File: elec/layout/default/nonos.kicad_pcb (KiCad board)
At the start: 4 copper layers, 45 x 122 mm, 75 parts, among them CN1 HRSHirose_DF40C_100DS_0_4V51, CN2 HRSHirose_DF40C_100DS_0_4V51, Q1 MOSFET, U1 STUSB4500QTR, U2 _Texas_Instruments_SN74LVC1G0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, U3 _Texas_Instruments_TAS5825MRH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, U4 _HCTL_HC_TYPE_C_24P_VS9_3_5A_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, U5 JST_Sales_America_B02B_XASK_1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, U6 JST_Sales_America_B02B_XASK_1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, U7 _Texas_Instruments_TPS56637RP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

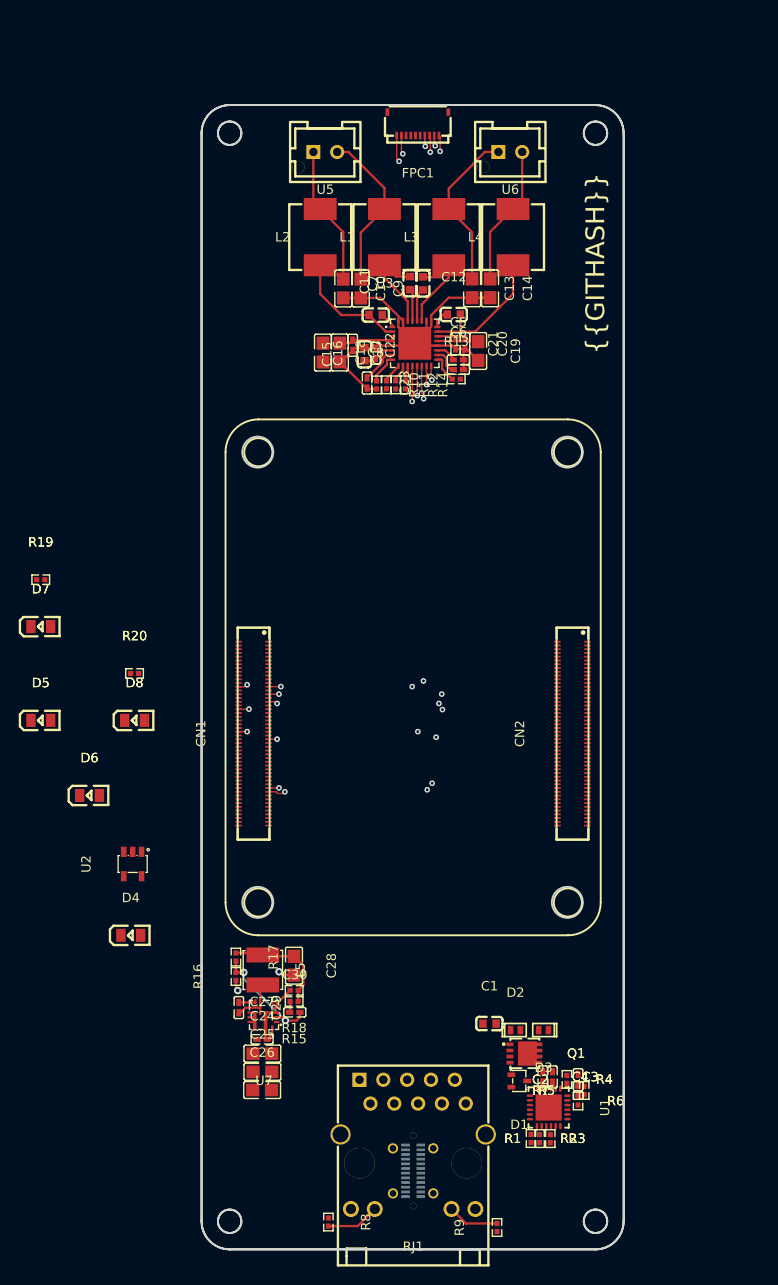
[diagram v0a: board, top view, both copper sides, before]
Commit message: layout 95%
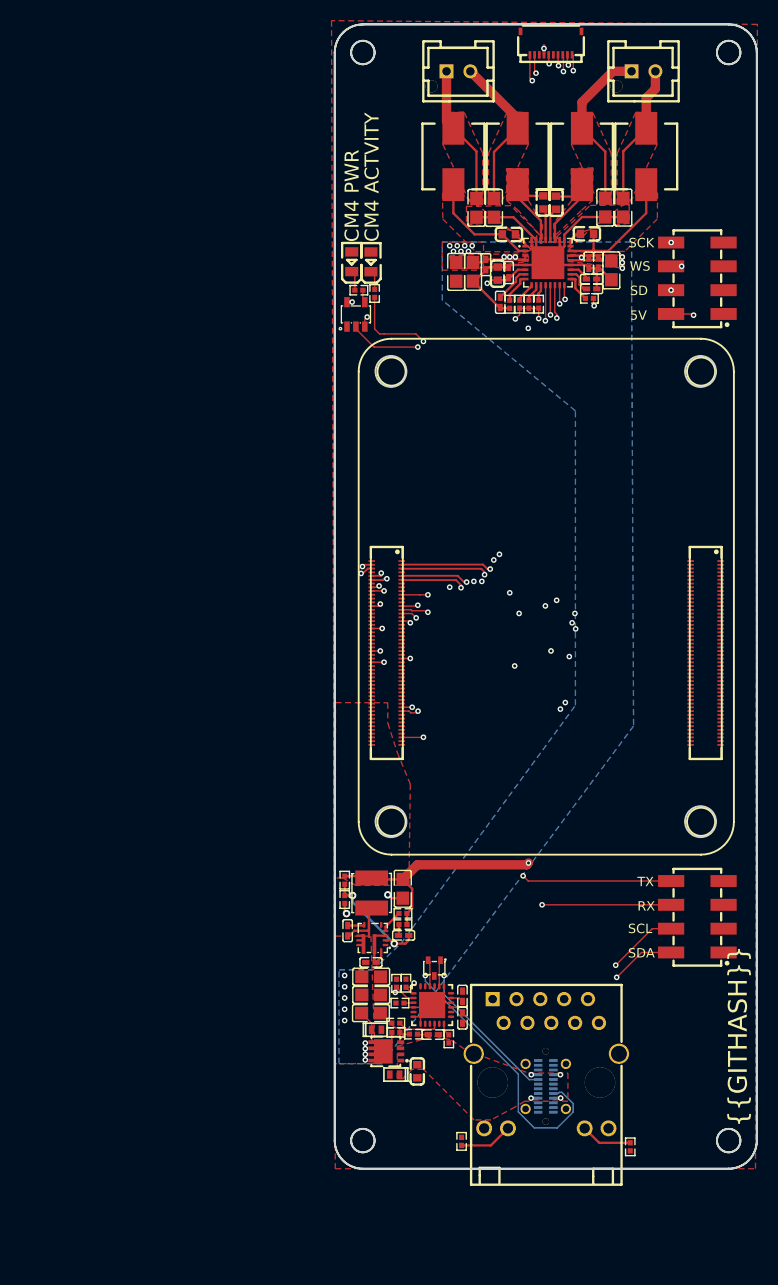
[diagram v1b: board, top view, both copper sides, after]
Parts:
- removed D6, D7, D8: , lcsc:LED0805-R-RD
- added HDR1: HCTL_PZ254_2_04_S, lcsc:HDR-SMD_8P-P2.54-V-M-R2-C4-LS7.4, F.Cu at (169.4, 130.9)
- added HDR2: HCTL_PZ254_2_04_S, lcsc:HDR-SMD_8P-P2.54-V-M-R2-C4-LS7.4, F.Cu at (169.4, 62.9)
- C2: value 100nF ±10% 16V X7R -> 1µF ±10% 25V X5R
- C4: value 1µF ±10% 25V X5R -> 100nF ±10% 16V X7R
- moved D4 76.2 mm to (134.6, 61.1), turned to 90 degrees
- moved U2 63.2 mm to (133.0, 66.7), turned to -90 degrees
- moved D5 59.1 mm to (132.6, 61.1), turned to 90 degrees
- moved R20 47.3 mm to (133.3, 64.1)
- moved R19 46.9 mm to (135.0, 64.5), turned to -90 degrees
- moved R3 22.5 mm to (137.3, 138.0), turned to 90 degrees
- moved R1 21.6 mm to (137.7, 140.1), turned to 0 degrees
- moved R2 21.3 mm to (138.3, 138.0), turned to 90 degrees
- moved R6 21.1 mm to (137.3, 142.3), turned to 0 degrees
- moved R5 21.0 mm to (137.3, 143.3), turned to 180 degrees
- moved R7 18.6 mm to (139.1, 143.5), turned to 0 degrees
- moved D3 17.8 mm to (135.2, 143.0), turned to 0 degrees
- moved U4 16.8 mm to (153.2, 149.0)
- moved C23 16.6 mm to (148.4, 65.4)
- moved R11 16.6 mm to (150.5, 65.6)
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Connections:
- net pd_controller.PD_CONTROLLER-signal renamed pd_controller.pd_controller-signal-1
- net pd_controller.PD_CONTROLLER-signal-1 renamed pd_controller.pd_controller-signal
- net pd_controller.PD_CONTROLLER.footprint.pins[18].net-net renamed pd_controller.pd_controller.footprint.pins[18].net-net
- net pins[40] renamed processor.hdi_b-pins[40]
- net pins[46] renamed processor-pins[46]-1
- net pins[49] renamed processor.hdi_b-pins[49]
- net processor-signal-8 renamed processor-pins[49]
- net processor.hdi_b-pins[23] renamed pins[23]
- net processor.hdi_b-pins[26] renamed pins[26]
- net processor.hdi_b-pins[28] renamed pins[28]
- C10 pad 1: net -> net-2
- C11 pad 1: amplifier-net-5 -> amplifier-net-3
- C11 pad 2: amplifier-net-4 -> amplifier-net-2
- C12 pad 1: amplifier-net-3 -> amplifier-net-7
- C12 pad 2: amplifier-net-1 -> amplifier-net
- C13 pad 1: net-3 -> net-1
- C14 pad 1: net-1 -> net
- C2 pad 1: pd_controller-net-4 -> GND
- C2 pad 2: VBUS -> VREG_1V2
- C23 pad 1: amplifier-net-7 -> amplifier-net-6
- C29 pad 1: regulator-net-4 -> regulator-net
- C29 pad 2: regulator-net-3 -> regulator-net-1
- C3 pad 2: VREG_1V2 -> VREG_2V7
- C30 pad 1: regulator-net-1 -> regulator-net-2
- C30 pad 2: regulator-net -> regulator-net-3
- C4 pad 1: GND -> pd_controller-net-3
- C4 pad 2: VREG_2V7 -> VBUS
- C6 pad 1: amplifier-net -> amplifier-net-1
- C7 pad 1: amplifier-net-6 -> amplifier-net-11
- C7 pad 2: amplifier-net-9 -> amplifier-net-8
- C8 pad 1: amplifier-net-2 -> amplifier-net-4
- C8 pad 2: amplifier-net-8 -> amplifier-net-5
- C9 pad 1: net-2 -> net-3
- CN1 pad 10: processor-net-3 -> processor-net-2
- CN1 pad 12: processor-pins[23] -> processor-signal
- CN1 pad 14: processor-signal-3 -> UART_TX
- CN1 pad 15: signal-7 -> signal-3
- CN1 pad 17: signal-5 -> signal-4
- CN1 pad 22: pins[43] -> processor-signal-3
- CN1 pad 23: processor-signal-6 -> pins[45]
- CN1 pad 24: processor-signal-7 -> processor-signal-2
- CN1 pad 27: signal-4 -> signal-5
- CN1 pad 28: signal-3 -> signal-2
- CN1 pad 29: signal-2 -> signal-1
- CN1 pad 73: processor-signal-5 -> UART_RX
- CN1 pad 75: processor-signal-2 -> pins[50]
- CN1 pad 77: processor-signal-1 -> processor-pins[46]
- CN1 pad 78: processor-pins[44]-1 -> processor-pins[44]
- CN1 pad 80: processor-signal -> processor-pins[40]
- CN1 pad 81: processor-signal-9 -> processor-signal-1
- CN1 pad 82: signal-6 -> signal
- CN1 pad 85: processor-signal-4 -> processor-signal-6
- CN1 pad 86: processor-pins[28] -> processor-signal-5
- CN1 pad 87: processor-pins[26] -> processor-signal-4
- CN2 pad 78: processor-pins[44] -> processor-pins[44]-1
- D4 pad 2: processor-net -> processor-net-3
- D5 pad 1: processor.power_1v8_led-anode -> VCC_3V3
- D5 pad 2: processor.power_1v8_led-cathode -> processor-net-1
- FPC1 pad 10: signal-6 -> signal
- FPC1 pad 7: signal-4 -> signal-5
- FPC1 pad 8: signal-5 -> signal-4
- FPC1 pad 9: signal-7 -> signal-3
- L1 pad 1: amplifier-net-9 -> amplifier-net-8
- L1 pad 2: net-2 -> net-3
- L2 pad 1: amplifier-net-8 -> amplifier-net-5
- L2 pad 2: net -> net-2
- L3 pad 1: amplifier-net-4 -> amplifier-net-2
- L3 pad 2: net-3 -> net-1
- L4 pad 1: amplifier-net-1 -> amplifier-net
- L4 pad 2: net-1 -> net
- L5 pad 2: regulator-net-3 -> regulator-net-1
- Q1 pad 1: pd_controller.VSINK_MOSFET.footprint.pins[0].net-net -> VBUS
- Q1 pad 2: pd_controller.VSINK_MOSFET.footprint.pins[1].net-net -> VBUS
- Q1 pad 4: pd_controller-net -> pd_controller-net-2
- Q1 pad 5: pd_controller.VSINK_MOSFET.footprint.pins[4].net-net -> VSINK_VCC
- Q1 pad 6: pd_controller.VSINK_MOSFET.footprint.pins[5].net-net -> VSINK_VCC
- Q1 pad 7: pd_controller.VSINK_MOSFET.footprint.pins[6].net-net -> VSINK_VCC
- Q1 pad 8: pd_controller.VSINK_MOSFET.footprint.pins[7].net-net -> VSINK_VCC
- R1 pad 2: pd_controller-net-3 -> pd_controller-net-1
- R10 pad 1: amplifier-net-11 -> amplifier-net-9
- R11 pad 1: signal-2 -> signal-1
- R12 pad 1: signal -> signal-7
- R13 pad 1: signal-3 -> signal-2
- R14 pad 1: signal-1 -> signal-6
- R15 pad 2: regulator-net-1 -> regulator-net-2
- R16 pad 2: regulator-net -> regulator-net-3
- R17 pad 2: regulator-net -> regulator-net-3
- R18 pad 2: regulator-net-2 -> regulator-net-4
- R19 pad 1: processor-net -> processor-net-3
- R19 pad 2: processor-net-1 -> processor-net-2
- R2 pad 1: I2C_SCL -> SCL
- R2 pad 2: hv -> VCC_3V3
- R20 pad 1: processor-net-2 -> processor-net-1
- R20 pad 2: processor-net-3 -> processor-net
- R3 pad 1: I2C_SDA -> SDA
- R3 pad 2: hv -> VCC_3V3
- R4 pad 2: pd_controller-net-2 -> pd_controller-net
- R5 pad 1: pd_controller-net -> pd_controller-net-2
- R6 pad 1: pd_controller-net -> pd_controller-net-2
- R6 pad 2: pd_controller-net-1 -> pd_controller-net-4
- R7 pad 1: pd_controller-net -> pd_controller-net-2
- R7 pad 2: pd_controller-net-4 -> pd_controller-net-3
- U1 pad 16: pd_controller-net-1 -> pd_controller-net-4
- U1 pad 18: pd_controller-net-2 -> pd_controller-net
- U1 pad 7: I2C_SCL -> SCL
- U1 pad 8: I2C_SDA -> SDA
- U1 pad 9: pd_controller-net-3 -> pd_controller-net-1
- U2 pad 4: processor-net-1 -> processor-net
- U3 pad 1: amplifier-net-2 -> amplifier-net-4
- U3 pad 10: signal -> signal-7
- U3 pad 11: signal-1 -> signal-6
- U3 pad 17: signal-3 -> signal-2
- U3 pad 18: amplifier-net -> amplifier-net-1
- U3 pad 2: amplifier-net-8 -> amplifier-net-5
- U3 pad 23: amplifier-net-1 -> amplifier-net
- U3 pad 24: amplifier-net-3 -> amplifier-net-7
- U3 pad 27: amplifier-net-4 -> amplifier-net-2
- U3 pad 28: amplifier-net-5 -> amplifier-net-3
- U3 pad 29: amplifier-net-6 -> amplifier-net-11
- U3 pad 30: amplifier-net-9 -> amplifier-net-8
- U3 pad 7: amplifier-net-7 -> amplifier-net-6
- U3 pad 8: amplifier-net-11 -> amplifier-net-9
- U3 pad 9: signal-2 -> signal-1
- U4 pad 25: usb_connector.connector-net -> GND
- U4 pad 26: usb_connector.connector-net -> GND
- U4 pad 27: usb_connector.connector-net -> GND
- U4 pad 28: usb_connector.connector-net -> GND
- U4 pad A1: usb_connector.connector-net-1 -> GND
- U4 pad A12: usb_connector.connector-net-1 -> GND
- U4 pad A4: VSINK_VCC -> VBUS
- U4 pad A6: usb_connector-net-1 -> usb_connector-net
- U4 pad A7: usb_connector-net -> usb_connector-net-1
- U4 pad A9: VSINK_VCC -> VBUS
- U4 pad B1: usb_connector.connector-net-1 -> GND
- U4 pad B12: usb_connector.connector-net-1 -> GND
- U4 pad B4: VSINK_VCC -> VBUS
- U4 pad B5: CC1 -> CC2
- U4 pad B6: usb_connector-net-1 -> usb_connector-net
- U4 pad B7: usb_connector-net -> usb_connector-net-1
- U4 pad B9: VSINK_VCC -> VBUS
- U5 pad 1: net -> net-2
- U5 pad 2: net-2 -> net-3
- U6 pad 1: net-3 -> net-1
- U6 pad 2: net-1 -> net
- U7 pad 2: regulator-net -> regulator-net-3
- U7 pad 4: regulator-net-2 -> regulator-net-4
- U7 pad 6: regulator-net-3 -> regulator-net-1
- U7 pad 7: regulator-net-4 -> regulator-net
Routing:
- net VCC_5V: track 11.8 -> 136.2 mm, vias 0 -> 4
- net signal-6: track 87.3 -> 1.70 mm, vias 3 -> 0
- net signal: track 1.91 -> 87.2 mm, vias 0 -> 3
- net signal-7: track 81.6 -> 1.91 mm, vias 3 -> 0
- net signal-3: track 3.34 -> 82.1 mm, vias 0 -> 3
- net ETH_LED_ACTIVITY: track 0.00 -> 78.5 mm, vias 0 -> 2
- net ETH_LED_LINK: track 0.00 -> 70.0 mm, vias 0 -> 2
- net ETH_P3_N: track 0.00 -> 69.5 mm, vias 0 -> 2
- net ETH_P3_P: track 0.00 -> 68.8 mm, vias 0 -> 2
- net ETH_P1_P: track 0.00 -> 67.0 mm, vias 0 -> 1
- net SDA: track 91.0 -> 157.3 mm, vias 4 -> 6
- net SCL: track 90.2 -> 154.3 mm, vias 4 -> 6
- net ETH_P2_N: track 0.00 -> 63.5 mm, vias 0 -> 2
- net ETH_P2_P: track 0.00 -> 60.3 mm, vias 0 -> 2
- net ETH_P1_N: track 0.00 -> 58.1 mm, vias 0 -> 1
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- added copper zone on F.Cu, net GND
- added copper zone on In2.Cu, net GND
- added copper zone on F.Cu, net VBUS
- added copper zone on F.Cu, net VCC_5V
- added copper zone on B.Cu, net VSINK_VCC
- added copper zone on F.Cu, net VSINK_VCC
- added copper zone on F.Cu, net amplifier-net
- added copper zone on F.Cu, net amplifier-net-2
- added copper zone on F.Cu, net amplifier-net-5
- added copper zone on F.Cu, net amplifier-net-8
- added copper zone on F.Cu, net net
- added copper zone on F.Cu, net net-1
- added copper zone on F.Cu, net net-2
- added copper zone on F.Cu, net net-3
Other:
- outline, holes or cut-outs redrawn
- board text added: "5V"
- board text added: "CM4 ACTVITY"
- board text added: "CM4 PWR"
- board text added: "NONOS"
- board text added: "RX"
- board text added: "SCK"
- board text added: "SCL"
- board text added: "SD"
- board text added: "SDA"
- board text added: "TX"
- board text added: "WS"

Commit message: layout complete
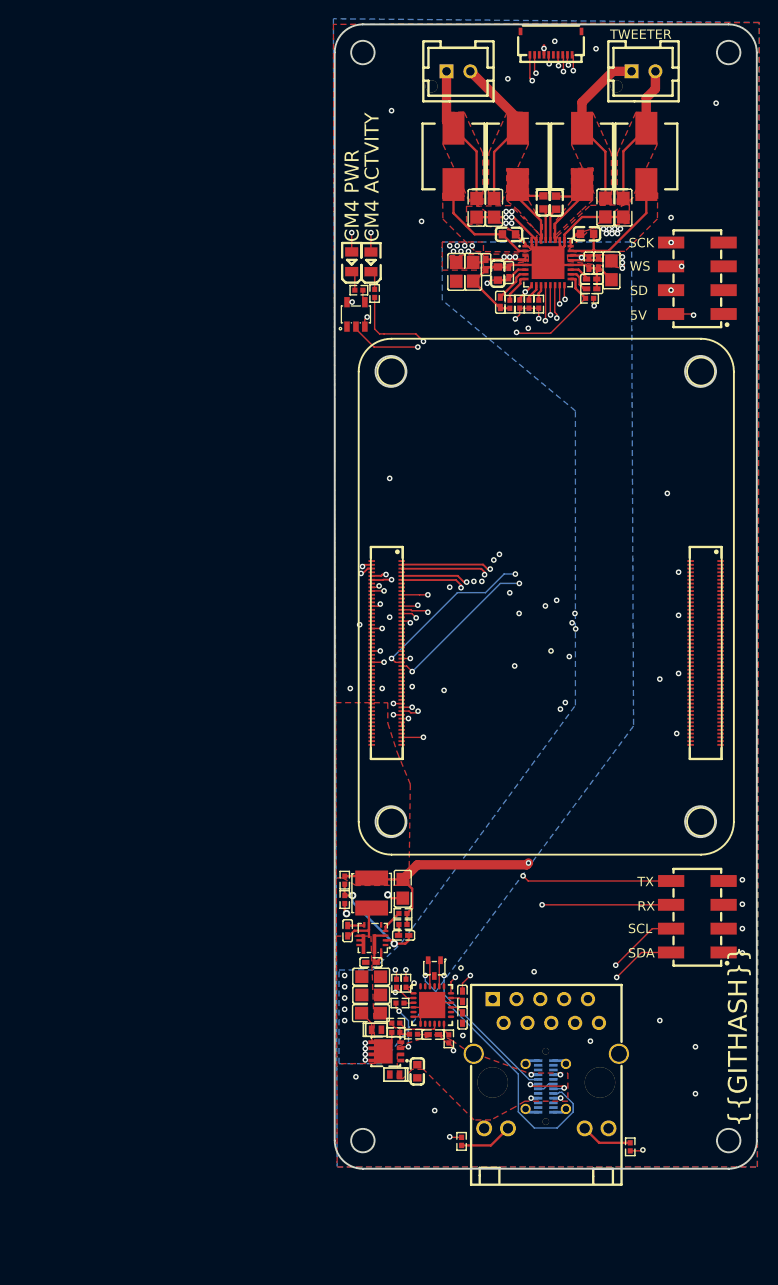
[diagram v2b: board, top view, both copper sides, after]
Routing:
- net signal-2: track 3.34 -> 56.3 mm, vias 0 -> 3
- net signal-1: track 2.11 -> 50.2 mm, vias 0 -> 3
- net VBUS: track 3.71 -> 22.1 mm, vias 4 -> 8
- net VCC_3V3: track 11.5 -> 22.8 mm, vias 6 -> 19
- net GND: track 68.5 -> 76.4 mm, vias 2 -> 45
- net usb_connector-net: track 0.00 -> 5.79 mm, vias 0 -> 2
- net usb_connector-net-1: track 0.00 -> 1.83 mm
- net VCC_5V: track 136.2 -> 136.7 mm
- added copper zone on B.Cu, net VCC_3V3
- added copper zone on In1.Cu, net VCC_3V3
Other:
- board text added: "TWEETER"
- board text added: "WOOFER"
